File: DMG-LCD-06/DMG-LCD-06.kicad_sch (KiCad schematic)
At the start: 46 parts, among them J1 Wire, J2 Wire, J3 Wire, J4 Wire, J5 Wire, Q1 2SA933SR, SW1 Left, SW2 Up, SW3 Down, SW4 Right, SW5 Select, SW6 Start, SW7 B, SW8 A, U1 IR3E02, U2 LH5076, U3 LH5077

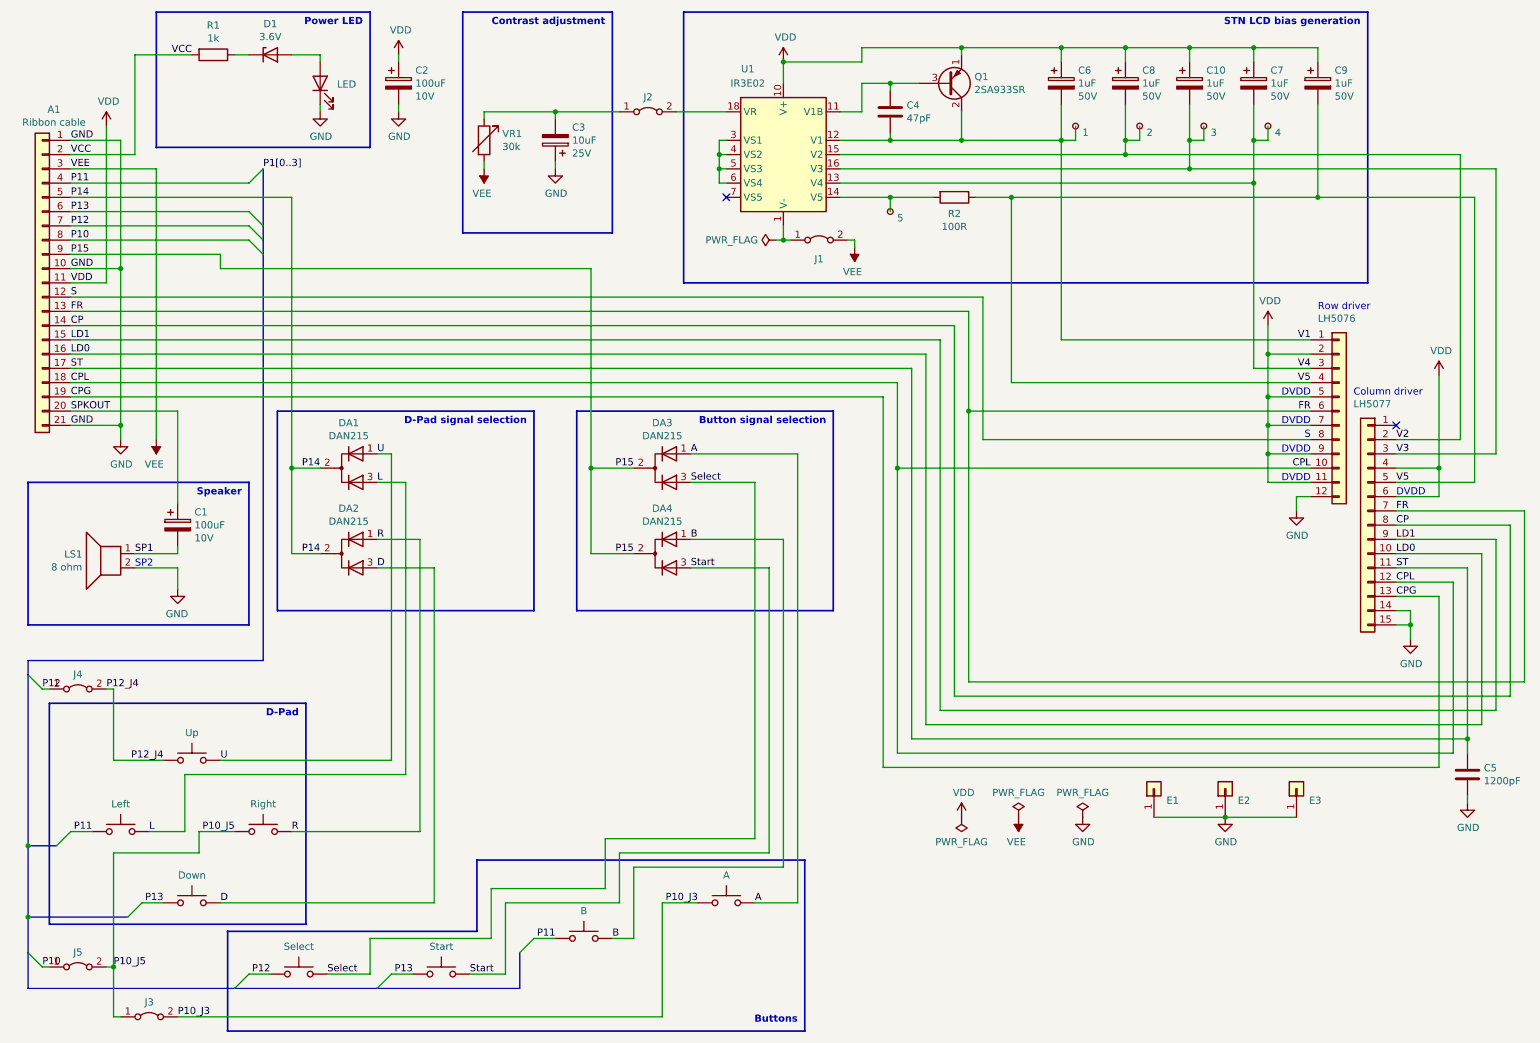
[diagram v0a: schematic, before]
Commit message: Update to latest KiCad
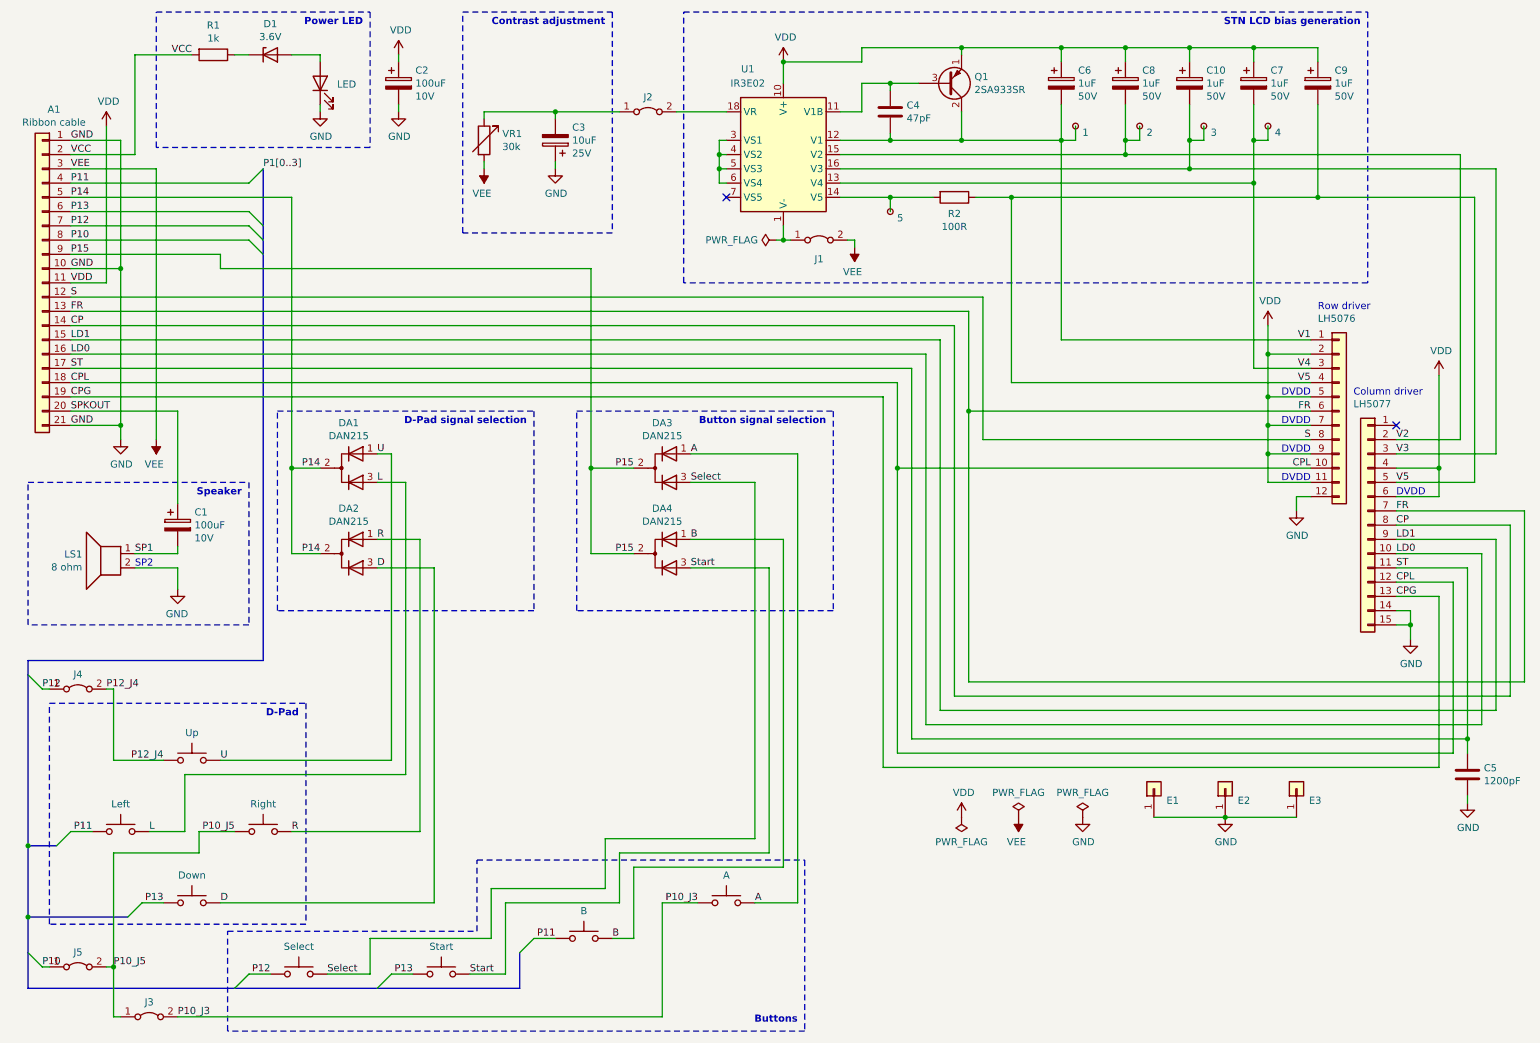
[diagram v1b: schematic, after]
